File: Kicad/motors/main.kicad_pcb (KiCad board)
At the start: 2 copper layers, 80 x 140 mm, 155 parts, among them K100 9V - 1A, K201 MOTOR 1, K202 MOTOR 2, K203 MOTOR 4, K204 MOTOR 3, K301 FRONT, K302 REAR, Q100 DMP2305U, Q101 DMP2305U, Q102 STN790A, Q301 BC846BS, Q302 BC846BS, U100 BQ2057W, U201 L298P, U202 SN74LVC1G19, U203 SN74LVC1G19, U204 L298P, U205 SN74LVC1G19, U206 SN74LVC1G19, U207 LM3480-50, U301 SN74LVC2G17, U302 SN74LVC2G17, U303 LM3480-33, X101 SYMBOL-MISC, X102 SYMBOL-MISC

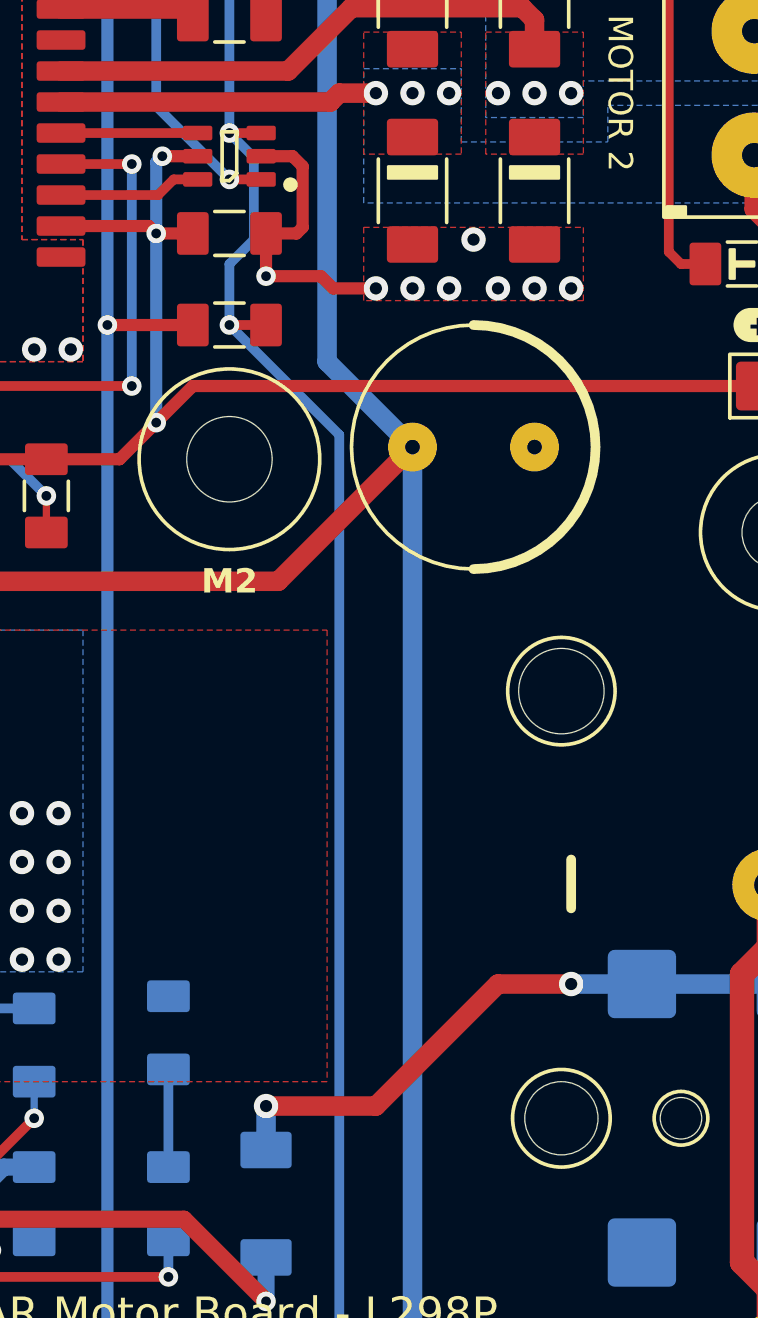
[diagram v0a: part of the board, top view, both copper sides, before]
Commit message: Up
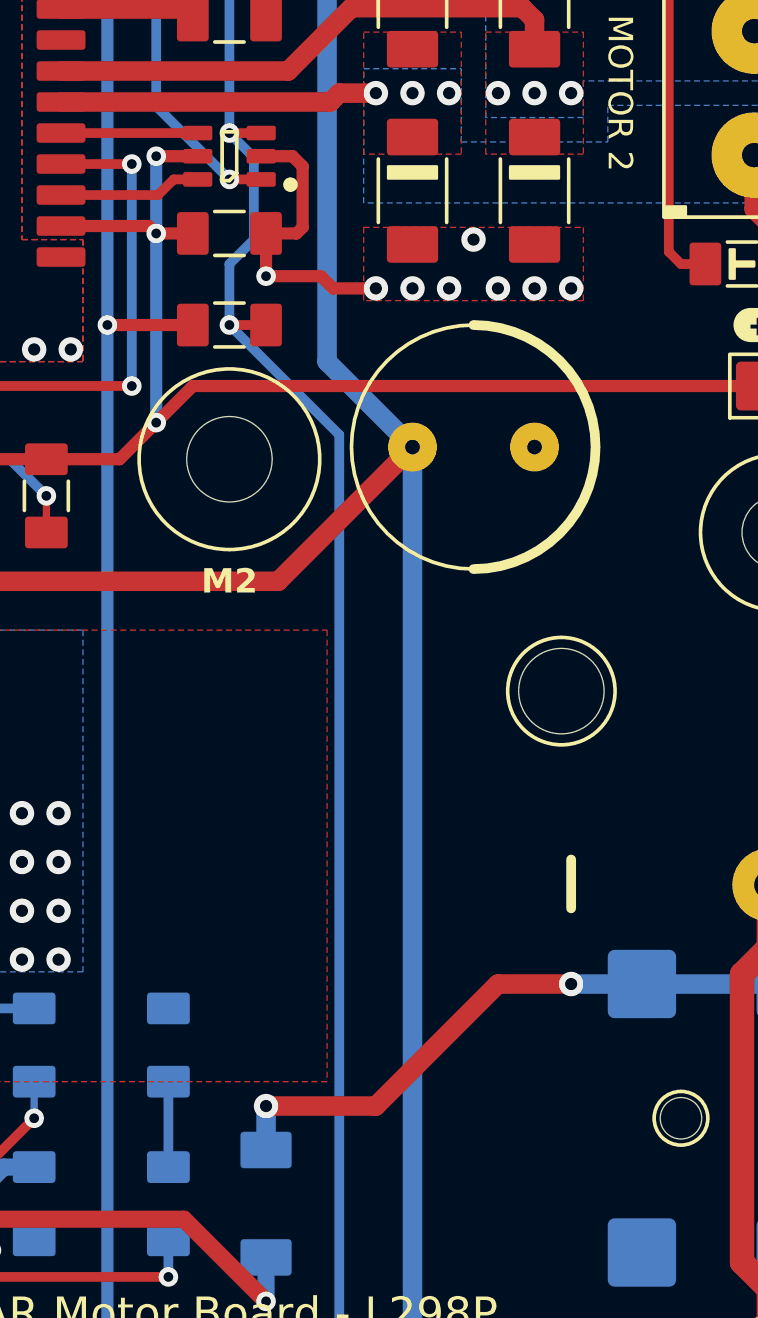
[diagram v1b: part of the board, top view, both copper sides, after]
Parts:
- moved LED100 0.50 mm to (100.5, 97.0)
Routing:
- net Net-(LED100-A): track 4.00 -> 3.50 mm
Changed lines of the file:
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@@
     (fp_circle (center 0 -27.6) (end 2 -27.6)
       (stroke (width 0.15) (type solid)) (fill none) (layer "B.SilkS"))
-    (fp_circle (center 0 27.6) (end 2 27.6)
-      (stroke (width 0.15) (type solid)) (fill none) (layer "B.SilkS"))
     (fp_circle (center 17.5 27.6) (end 19.7 27.6)
       (stroke (width 0.15) (type solid)) (fill none) (layer "B.SilkS"))
@@
     (fp_circle (center 0 -27.6) (end 2 -27.6)
       (stroke (width 0.15) (type solid)) (fill none) (layer "F.SilkS"))
-    (fp_circle (center 0 27.6) (end 2 27.6)
-      (stroke (width 0.15) (type solid)) (fill none) (layer "F.SilkS"))
     (fp_circle (center 17.5 27.6) (end 19.7 27.6)
       (stroke (width 0.15) (type solid)) (fill none) (layer "F.SilkS"))
@@
     (fp_circle (center 0 -27.6) (end 2 -27.6)
       (stroke (width 0.1) (type solid)) (fill none) (layer "F.Fab"))
-    (fp_circle (center 0 27.6) (end 2 27.6)
-      (stroke (width 0.1) (type solid)) (fill none) (layer "F.Fab"))
     (fp_circle (center 17.5 27.6) (end 19.7 27.6)
       (stroke (width 0.1) (type solid)) (fill none) (layer "F.Fab"))
@@
     (pad "" np_thru_hole circle (at -17.5 36.1 90) (size 1.6 1.6) (drill 1.6) (layers "F&B.Cu" "*.Mask"))
     (pad "" np_thru_hole circle (at 0 -27.6 90) (size 3 3) (drill 3) (layers "F&B.Cu" "*.Mask"))
-    (pad "" np_thru_hole circle (at 0 27.6 90) (size 3 3) (drill 3) (layers "F&B.Cu" "*.Mask"))
     (pad "" np_thru_hole circle (at 17.5 27.6 90) (size 3.5 3.5) (drill 3.5) (layers "F&B.Cu" "*.Mask"))
     (pad "1" thru_hole circle (at 9.56 36.1 90) (size 3 3) (drill 1.2) (layers "*.Cu" "*.Mask")
@@
   )
   (footprint "tronixio:LED-SMD-1206" (layer "B.Cu")
-    (at 100.5 96.5 -90)
+    (at 100.5 97 -90)
     (property "Mouser" "604-APT3216LSECKJ3RV")
     (property "Sheetfile" "main.kicad_sch")
@@
     (effects (font (size 1 1) (thickness 0.15)) (justify mirror))
   )
-  (gr_text "Charge" (at 102.5 96.5 90) (layer "B.SilkS")
+  (gr_text "Charge" (at 102.5 97 90) (layer "B.SilkS")
     (effects (font (size 1 1) (thickness 0.15)) (justify mirror))
   )
@@
   (segment (start 71.5 153) (end 71.5 134) (width 0.8) (layer "B.Cu") (net 2))
   (segment (start 70 50) (end 69 50) (width 0.8) (layer "B.Cu") (net 2))
-  (segment (start 82 93.5) (end 55.96 93.5) (width 0.8) (layer "F.Cu") (net 3))
-  (segment (start 55.96 93.5) (end 52.9 90.44) (width 0.8) (layer "F.Cu") (net 3))
   (segment (start 57 72) (end 55 70) (width 0.8) (layer "F.Cu") (net 3))
   (segment (start 57 78) (end 57 72) (width 0.8) (layer "F.Cu") (net 3))
+  (segment (start 82 93.5) (end 55.96 93.5) (width 0.8) (layer "F.Cu") (net 3))
   (segment (start 52.9 90.44) (end 52.9 82.1) (width 0.8) (layer "F.Cu") (net 3))
   (segment (start 52.9 82.1) (end 57 78) (width 0.8) (layer "F.Cu") (net 3))
   (segment (start 55 70) (end 52.5 70) (width 0.8) (layer "F.Cu") (net 3))
+  (segment (start 55.96 93.5) (end 52.9 90.44) (width 0.8) (layer "F.Cu") (net 3))
   (via (at 82 89.5) (size 1) (drill 0.5) (layers "F.Cu" "B.Cu") (free) (net 3))
   (via (at 94.5 87.5) (size 1) (drill 0.5) (layers "F.Cu" "B.Cu") (free) (net 3))
@@
   (segment (start 78 67.75) (end 78 69.5) (width 0.5) (layer "F.Cu") (net 4))
   (segment (start 92.5 72) (end 92.5 73) (width 0.5) (layer "F.Cu") (net 4))
-  (segment (start 100.2505 60.585) (end 100.25 60.5845) (width 0.5) (layer "F.Cu") (net 4))
   (segment (start 78.5 132.5) (end 80.75 130.25) (width 0.5) (layer "F.Cu") (net 4))
   (segment (start 98.5 73) (end 95.5 73) (width 0.5) (layer "F.Cu") (net 4))
   (segment (start 76.5 136.25) (end 78.5 136.25) (width 0.5) (layer "F.Cu") (net 4))
+  (segment (start 101.7 60.585) (end 100.0005 60.585) (width 0.5) (layer "F.Cu") (net 4))
   (segment (start 91.3 73) (end 92.5 73) (width 0.5) (layer "F.Cu") (net 4))
   (segment (start 76.3 64.5) (end 78 64.5) (width 0.5) (layer "F.Cu") (net 4))
-  (segment (start 101.7 60.585) (end 100.2505 60.585) (width 0.5) (layer "F.Cu") (net 4))
   (segment (start 89.95 73.3) (end 91 73.3) (width 0.5) (layer "F.Cu") (net 4))
   (segment (start 80.75 130.25) (end 98.25 130.25) (width 0.5) (layer "F.Cu") (net 4))
   (segment (start 79.75 71.25) (end 91.75 71.25) (width 0.5) (layer "F.Cu") (net 4))
+  (segment (start 100.0005 60.585) (end 100 60.5845) (width 0.5) (layer "F.Cu") (net 4))
   (segment (start 78 69.5) (end 79.75 71.25) (width 0.5) (layer "F.Cu") (net 4))
   (segment (start 78.5 136.25) (end 78.5 132.5) (width 0.5) (layer "F.Cu") (net 4))
@@
   (via (at 78 64.5) (size 0.8) (drill 0.4) (layers "F.Cu" "B.Cu") (net 4))
   (via (at 100.25 135.5) (size 0.8) (drill 0.4) (layers "F.Cu" "B.Cu") (net 4))
-  (via (at 100.25 60.5845) (size 0.8) (drill 0.4) (layers "F.Cu" "B.Cu") (net 4))
+  (via (at 100 60.5845) (size 0.8) (drill 0.4) (layers "F.Cu" "B.Cu") (net 4))
   (via (at 78.5 136.25) (size 0.8) (drill 0.4) (layers "F.Cu" "B.Cu") (net 4))
   (via (at 100 63.75) (size 0.8) (drill 0.4) (layers "F.Cu" "B.Cu") (net 4))
   (segment (start 78 67.75) (end 78 64.5) (width 0.5) (layer "B.Cu") (net 4))
-  (segment (start 100 63.75) (end 100 60.8345) (width 0.5) (layer "B.Cu") (net 4))
   (segment (start 100.25 135.5) (end 100.25 132.25) (width 0.5) (layer "B.Cu") (net 4))
   (segment (start 78.5 126) (end 74 121.5) (width 0.5) (layer "B.Cu") (net 4))
@@
   (segment (start 78 75.5) (end 78 67.75) (width 0.5) (layer "B.Cu") (net 4))
   (segment (start 74 121.5) (end 74 79.5) (width 0.5) (layer "B.Cu") (net 4))
+  (segment (start 100 63.75) (end 100 60.5845) (width 0.5) (layer "B.Cu") (net 4))
   (segment (start 78.5 136.25) (end 78.5 126) (width 0.5) (layer "B.Cu") (net 4))
   (segment (start 74 79.5) (end 78 75.5) (width 0.5) (layer "B.Cu") (net 4))
-  (segment (start 100 60.8345) (end 100.25 60.5845) (width 0.5) (layer "B.Cu") (net 4))
   (segment (start 125.1 107) (end 125.1 109.56) (width 1) (layer "F.Cu") (net 5))
   (segment (start 124 94.1) (end 125.1 93) (width 1) (layer "F.Cu") (net 5))
@@
   (segment (start 101.5 151) (end 101.5 147.5) (width 0.4) (layer "B.Cu") (net 33))
   (segment (start 96.5 164.5) (end 96.5 156) (width 0.4) (layer "B.Cu") (net 33))
-  (segment (start 100.5 102) (end 100.5 98) (width 0.4) (layer "B.Cu") (net 34))
+  (segment (start 100.5 102) (end 100.5 98.5) (width 0.4) (layer "B.Cu") (net 34))
   (segment (start 57.5 165.5) (end 67.5 165.5) (width 0.4) (layer "F.Cu") (net 35))
   (segment (start 56.5 51) (end 55.5 51) (width 0.4) (layer "F.Cu") (net 36))
